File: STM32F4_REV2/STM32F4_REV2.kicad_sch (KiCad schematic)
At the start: 0 parts

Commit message: Uploading the PCB files
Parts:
- added C1, C2: 2u2, Package_QFP:LQFP-64_10x10mm_P0.5mm, symbol Device:C_Small
- added R1: 10k, Resistor_THT:R_Array_SIP4, symbol Device:R_Small
- added SW1: SW_SPDT, Button_Switch_SMD:SW_SPST_CK_KMS2xxGP, symbol Switch:SW_SPDT
- added U1: STM32F405RGT6, Package_QFP:LQFP-64_10x10mm_P0.5mm, symbol MCU_ST_STM32F4:STM32F405RGTx
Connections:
- new net: C2.1, U1.31 (VCAP_1)
- new net: R1.2, SW1.2 (B)
- new net: C1.1, U1.47 (VCAP_2)
- new net +3.3V: SW1.1 (A), U1.1 (VBAT), U1.19 (VDD), U1.32 (VDD), U1.48 (VDD), U1.64 (VDD)
- new net +3.3VA: U1.13 (VDDA)
- new net BOOT0: R1.1, U1.60 (BOOT0)
- new net GND: C1.2, C2.2, SW1.3 (C), U1.12 (VSSA), U1.18 (VSS), U1.63 (VSS)
- new net HSE_IN: U1.5 (PH0)
- new net HSE_OUT: U1.6 (PH1)
- new net NRST: U1.7 (NRST)
- new net SWDIO: U1.46 (PA13)
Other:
- company: (none) -> Quanttronix
- title: (none) -> STM32F4 Board

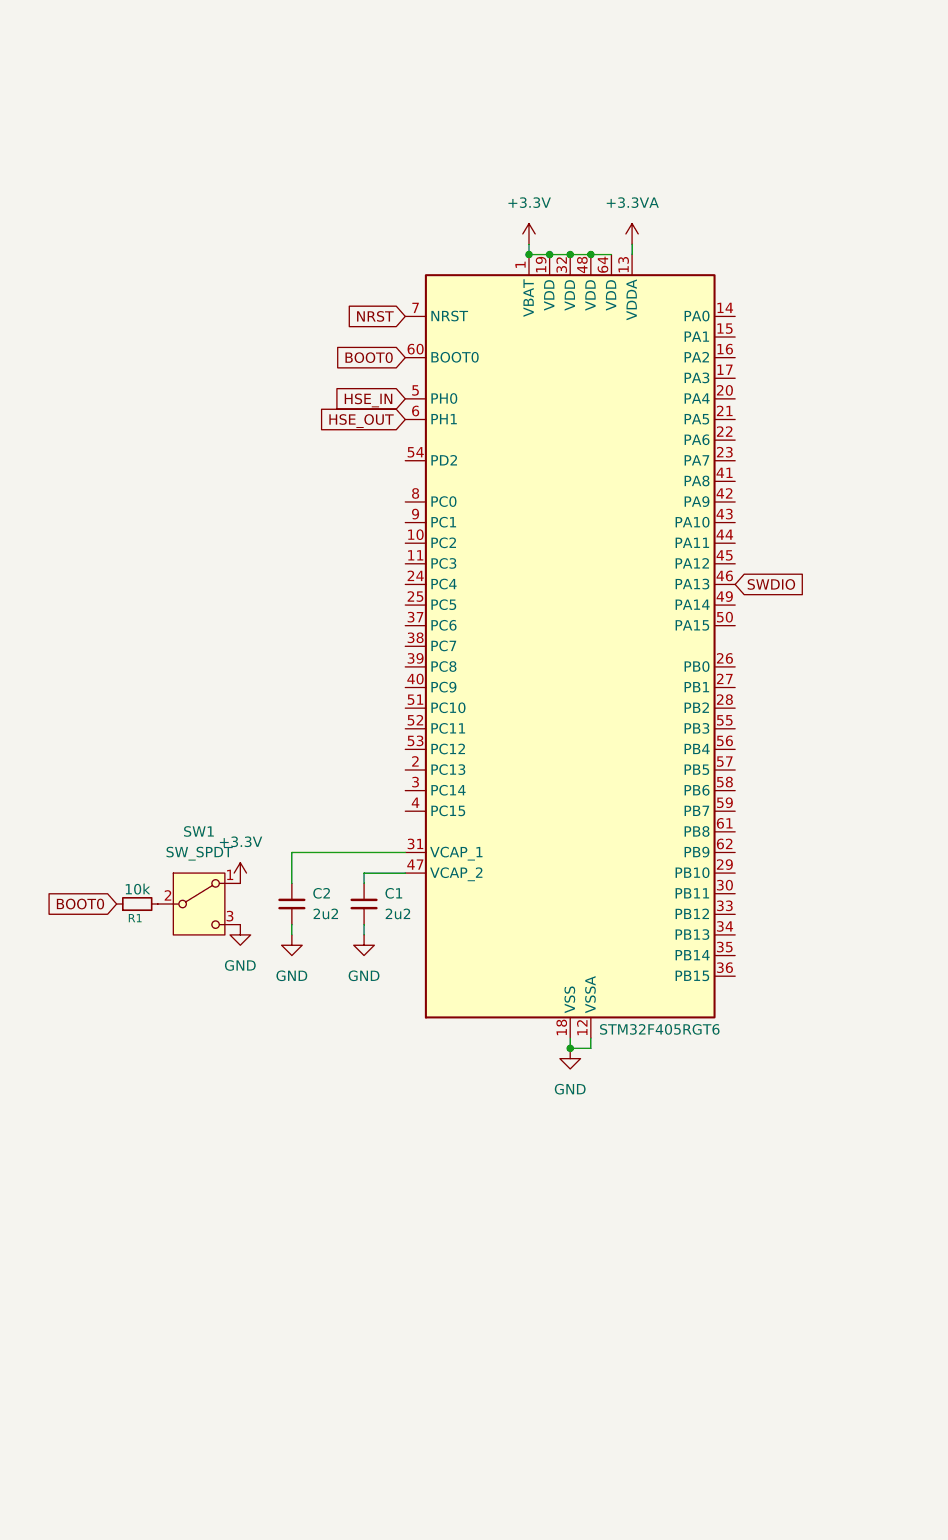
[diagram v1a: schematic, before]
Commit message: Updating the files
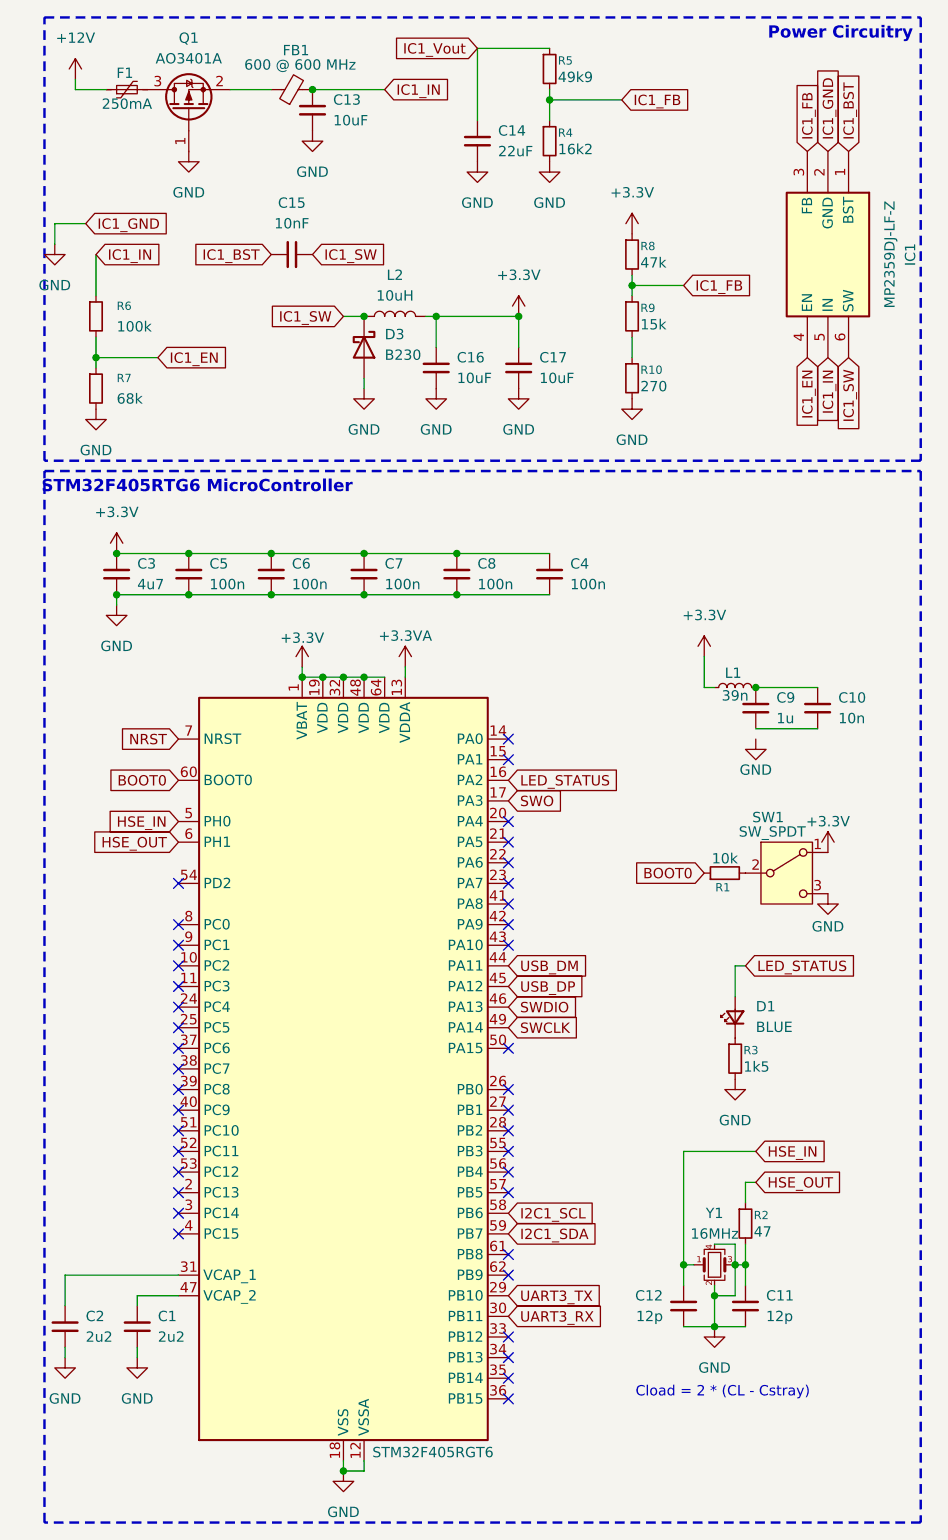
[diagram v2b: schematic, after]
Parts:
- added C10: 10n, symbol Device:C_Small
- added C11, C12: 12p, symbol Device:C_Small
- added C13, C16, C17: 10uF, symbol Device:C_Small
- added C14: 22uF, symbol Device:C_Small
- added C15: 10nF, symbol Device:C_Small
- added C3: 4u7, symbol Device:C_Small
- added C4, C5, C6, C7, C8: 100n, symbol Device:C_Small
- added C9: 1u, symbol Device:C_Small
- added D1: BLUE, symbol Device:LED_Small
- added D3: B230, Diode_SMD:D_SMB, symbol Diode:B230
- added F1: 250mA, symbol Device:Polyfuse_Small
- added FB1: 600 @ 600 MHz, Package_LCC:PLCC-84_29.3x29.3mm_P1.27mm, symbol Device:FerriteBead_Small
- added IC1: MP2359DJ-LF-Z, symbol SchmilliKiCADLibrary:MP2359DJ-LF-Z
- added L1: 39n, symbol Device:L_Small
- added L2: 10uH, Package_SON:WSON-8-1EP_6x5mm_P1.27mm_EP3.4x4mm, symbol Device:L
- added Q1: AO3401A, Package_TO_SOT_SMD:SOT-23, symbol Transistor_FET:AO3401A
- added R10: 270, symbol Device:R_Small
- added R2: 47, symbol Device:R_Small
- added R3: 1k5, symbol Device:R_Small
- added R4: 16k2, symbol Device:R_Small
- added R5: 49k9, symbol Device:R_Small
- added R6: 100k, symbol Device:R_Small
- added R7: 68k, symbol Device:R_Small
- added R8: 47k, symbol Device:R_Small
- added R9: 15k, symbol Device:R_Small
- added Y1: 16MHz, symbol Device:Crystal_GND24_Small
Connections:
- net +3.3V: now also C16.1, C17.1, C3.1, C4.1, C5.1, C6.1, C7.1, C8.1, L1.1, L2.2, R8.1
- net GND: now also C11.1, C11.2, C12.2, C13.2, C14.2, C16.2, C17.2, C3.2, C4.2, C5.2, C6.2, C7.2, C8.2, D3.2 (A), IC1.2 (GND), Q1.1 (G), R10.2, R2.2, R3.2, R4.2, R7.2, Y1.2 (G), Y1.3, Y1.4 (G)
- net HSE_IN: now also C12.1, Y1.1
- net HSE_OUT: now also R2.1
- net LED_STATUS: now reaches U1.16 (PA2)
- net LED_STATUS: now also D1.2 (A)
- net SWO: now reaches U1.17 (PA3)
- net UART3_TX: now reaches U1.29 (PB10)
- net UART3_RX: now reaches U1.30 (PB11)
- net USB_DM: now reaches U1.44 (PA11)
- net USB_DP: now reaches U1.45 (PA12)
- net SWCLK: now reaches U1.49 (PA14)
- net I2C1_SCL: now reaches U1.58 (PB6)
- net I2C1_SDA: now reaches U1.59 (PB7)
- new net: D1.1 (K), R3.1
- new net: C10.1, C9.1, L1.2
- new net: C10.2, C9.2
- new net: FB1.1, Q1.2 (S)
- new net: F1.2, Q1.3 (D)
- new net: R10.1, R9.2
- new net +12V: F1.1
- new net IC1_BST: C15.1, IC1.1 (BST)
- new net IC1_EN: IC1.4 (EN), R6.2, R7.1
- new net IC1_FB: IC1.3 (FB), R4.1, R5.2, R8.2, R9.1
- new net IC1_IN: C13.1, FB1.2, IC1.5 (IN), R6.1
- new net IC1_SW: C15.2, D3.1 (K), IC1.6 (SW), L2.1
- new net IC1_Vout: C14.1, R5.1
- no-connect marks 0 -> 39
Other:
- note added: "Cload = 2 * (CL - Cstray)"
- note added: "Power Circuitry"
- note added: "STM32F405RTG6 MicroController"
- moved on the sheet: C1, C2, R1, SW1

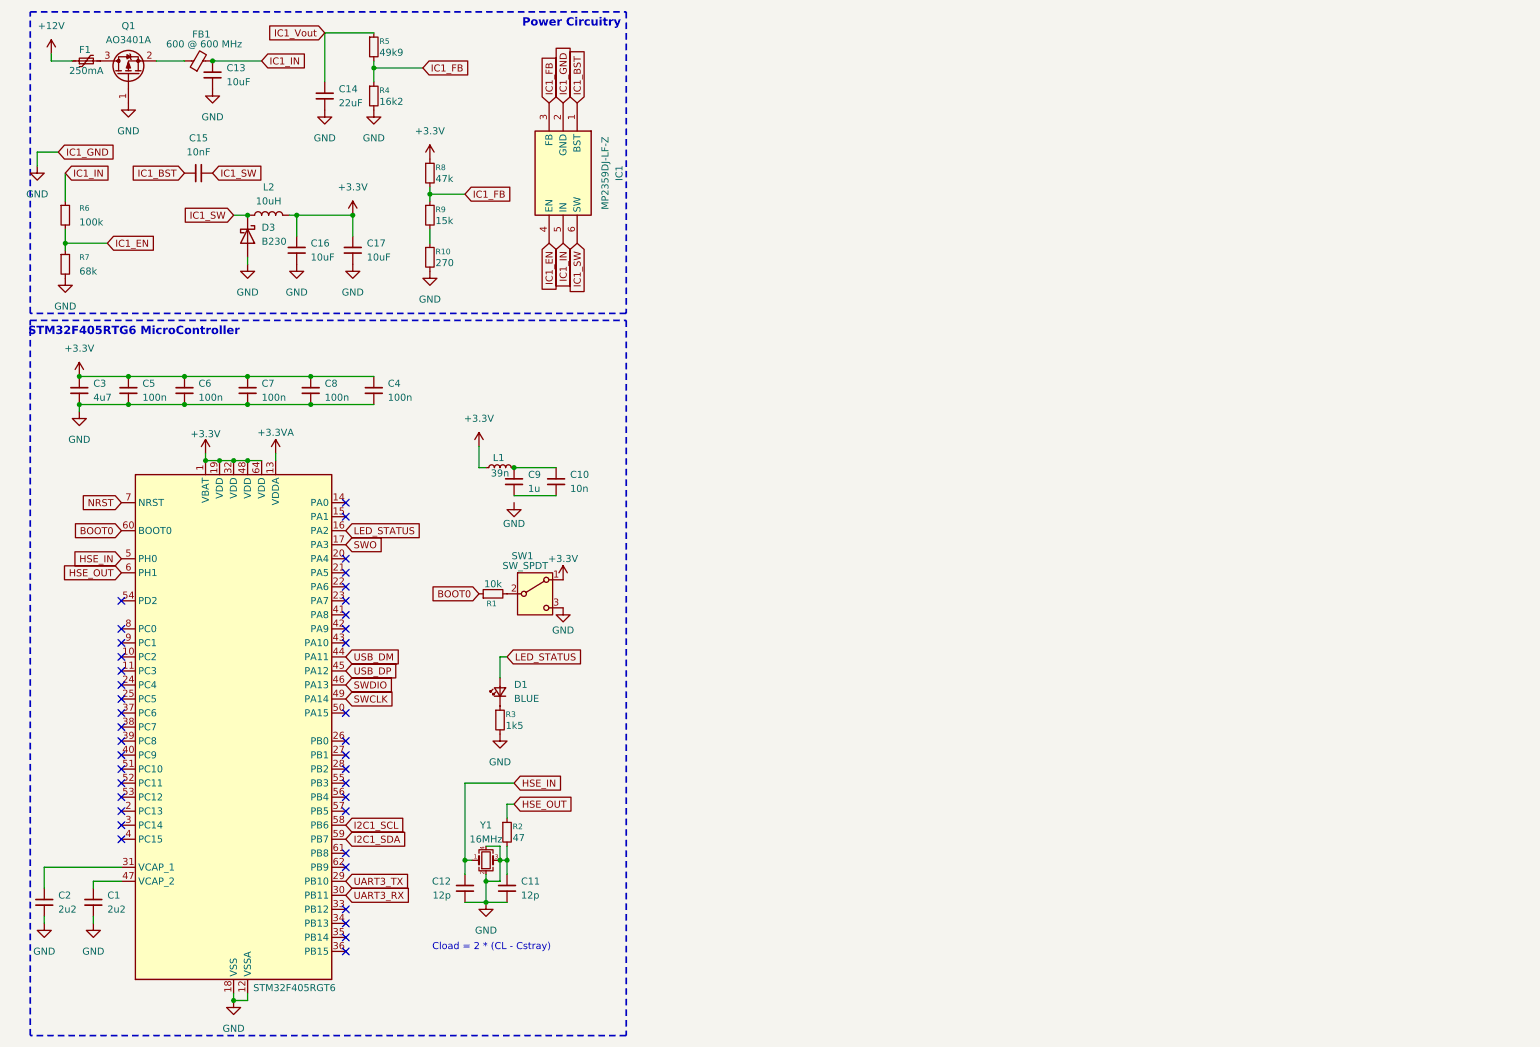
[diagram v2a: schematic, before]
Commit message: Uploading the PCB files
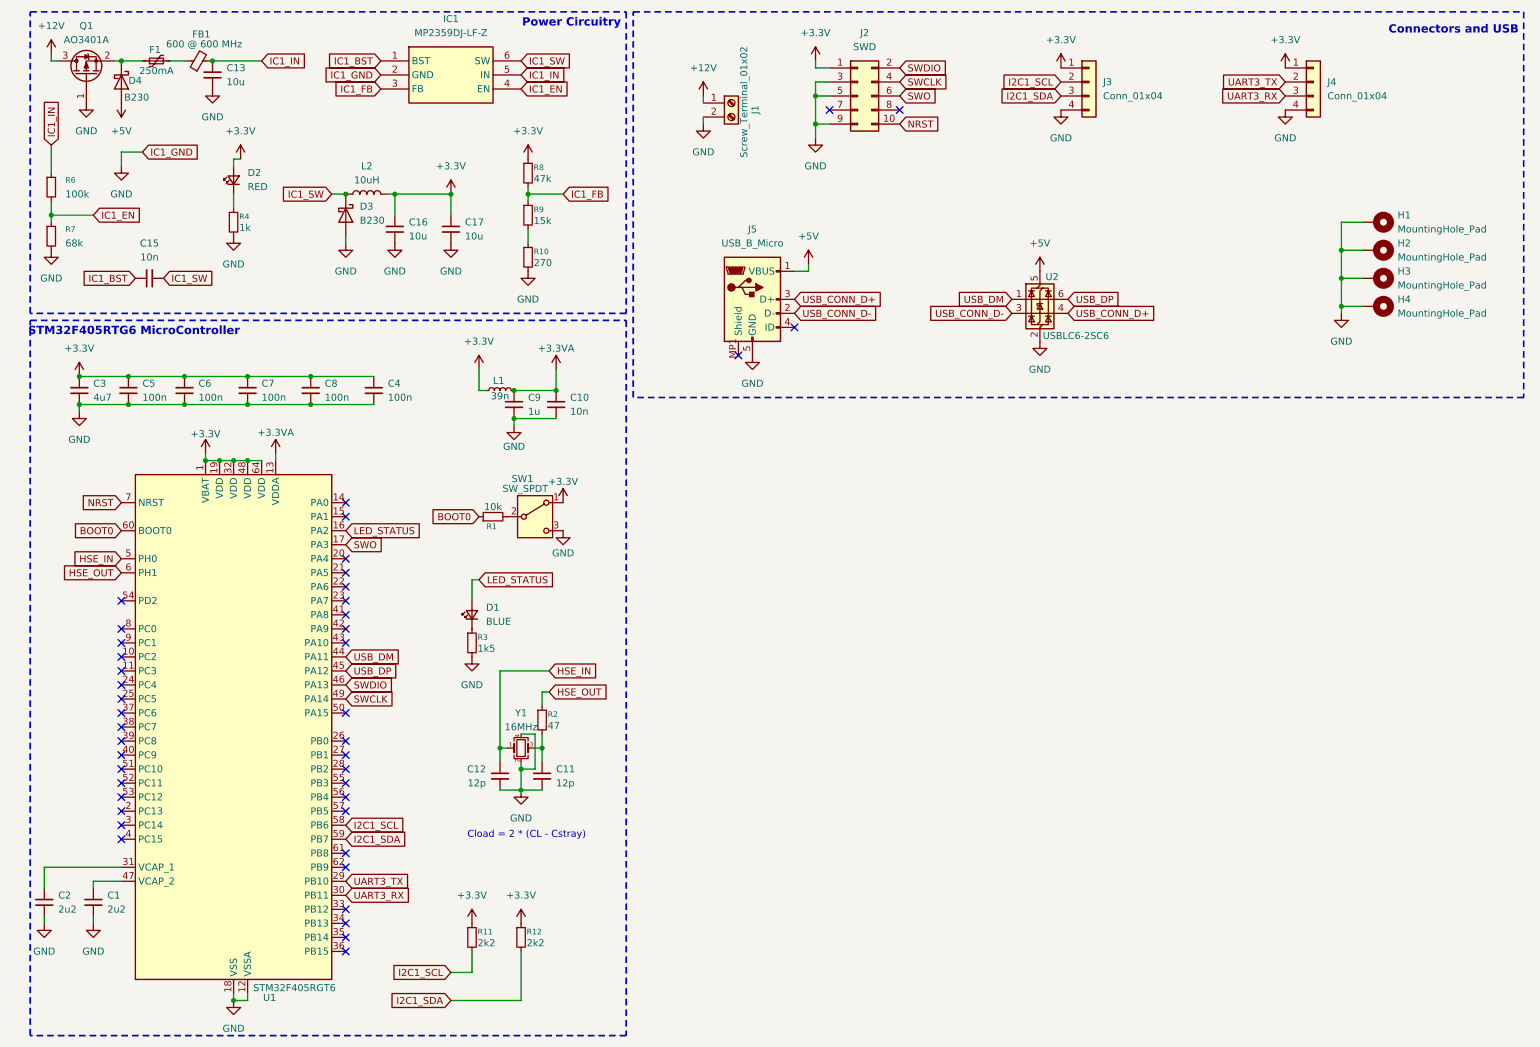
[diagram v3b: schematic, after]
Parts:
- removed C14: 22uF, symbol Device:C_Small
- removed IC1: MP2359DJ-LF-Z, symbol SchmilliKiCADLibrary:MP2359DJ-LF-Z
- removed R5: 49k9, symbol Device:R_Small
- added D2: RED, LED_SMD:LED_0603_1608Metric, symbol Device:LED_Small
- added D4: B230, Diode_SMD:D_SOD-123, symbol Diode:B230
- added H1, H2, H3, H4: MountingHole_Pad, MountingHole:MountingHole_4.3mm_M4_Pad_Via, symbol Mechanical:MountingHole_Pad
- added IC1: MP2359DJ-LF-Z, DownloadedLib:MP2359DJ-LF-Z, symbol DownloadedLib:MP2359DJ-LF-Z
- added J1: Screw_Terminal_01x02, TerminalBlock_Phoenix:TerminalBlock_Phoenix_PT-1,5-2-3.5-H_1x02_P3.50mm_Horizontal, symbol Connector:Screw_Terminal_01x02
- added J2: SWD, Connector_PinHeader_1.27mm:PinHeader_2x05_P1.27mm_Vertical_SMD, symbol Connector_Generic:Conn_02x05_Odd_Even
- added J3, J4: Conn_01x04, Connector_Molex:Molex_PicoBlade_53048-0410_1x04_P1.25mm_Horizontal, symbol Connector_Generic:Conn_01x04
- added J5: USB_B_Micro, DownloadedLib:101181930001LF, symbol Connector:USB_B_Micro
- added R11, R12: 2k2, Resistor_SMD:R_0402_1005Metric, symbol Device:R_Small
- added U2: USBLC6-2SC6, Package_TO_SOT_SMD:SOT-23-6, symbol Power_Protection:USBLC6-2SC6
- C1, C2: footprint Package_QFP:LQFP-64_10x10mm_P0.5mm -> Capacitor_SMD:C_0603_1608Metric
- C10, C11, C12, C4, C5, C6, C7, C8, C9: footprint (none) -> Capacitor_SMD:C_0402_1005Metric
- C13, C16, C17: value 10uF -> 10u; footprint (none) -> Capacitor_SMD:C_1206_3216Metric
- C15: value 10nF -> 10n; footprint (none) -> Capacitor_SMD:C_0603_1608Metric
- C3: footprint (none) -> Capacitor_SMD:C_0603_1608Metric
- D1: footprint (none) -> LED_SMD:LED_0603_1608Metric
- D3: footprint Diode_SMD:D_SMB -> Diode_SMD:D_SOD-123
- F1: footprint (none) -> Fuse:Fuse_1206_3216Metric
- FB1: footprint Package_LCC:PLCC-84_29.3x29.3mm_P1.27mm -> Capacitor_SMD:C_0805_2012Metric
- L1: footprint (none) -> Inductor_SMD:L_0402_1005Metric
- L2: footprint Package_SON:WSON-8-1EP_6x5mm_P1.27mm_EP3.4x4mm -> Inductor_SMD:L_Sunlord_MWSA0518S
- R1: footprint Resistor_THT:R_Array_SIP4 -> Resistor_SMD:R_0402_1005Metric
- R10, R3, R6, R7, R8, R9: footprint (none) -> Resistor_SMD:R_0603_1608Metric
- R2: footprint (none) -> Resistor_SMD:R_0402_1005Metric
- R4: value 16k2 -> 1k; footprint (none) -> Resistor_SMD:R_0603_1608Metric
- SW1: footprint Button_Switch_SMD:SW_SPST_CK_KMS2xxGP -> Button_Switch_SMD:SW_SPDT_PCM12
- Y1: footprint (none) -> Crystal:Crystal_SMD_3225-4Pin_3.2x2.5mm
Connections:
- net +12V: now also Q1.3 (D), J1.1 (Pin_1); no longer F1.1
- net +3.3V: now also D2.2 (A), J2.1 (Pin_1), J3.1 (Pin_1), J4.1 (Pin_1), R11.1, R12.1
- net +3.3VA: now also C10.1, C9.1, L1.2
- net GND: now also C10.2, C9.2, H1.1, H2.1, H3.1, H4.1, IC1.2 (GND), J1.2 (Pin_2), J2.3 (Pin_3), J2.5 (Pin_5), J2.9 (Pin_9), J3.4 (Pin_4), J4.4 (Pin_4), J5.5 (GND), U2.2 (GND); no longer C11.1, R2.2, Y1.3
- net I2C1_SCL: now also J3.2 (Pin_2), R11.2
- net I2C1_SDA: now also J3.3 (Pin_3), R12.2
- net IC1_BST: now also IC1.1 (BST)
- net IC1_EN: now also IC1.4 (EN)
- net IC1_FB: now also IC1.3 (FB); no longer R4.1
- net IC1_IN: now also IC1.5 (IN)
- net IC1_SW: now also IC1.6 (SW)
- net NRST: now also J2.10 (Pin_10)
- net SWCLK: now also J2.4 (Pin_4)
- net SWDIO: now also J2.2 (Pin_2)
- net SWO: now also J2.6 (Pin_6)
- net UART3_RX: now also J4.3 (Pin_3)
- net UART3_TX: now also J4.2 (Pin_2)
- net USB_DM: now also U2.1 (I/O1)
- net USB_DP: now also U2.6 (I/O1)
- net at Q1.2 (S): now also F1.1, D4.1 (K); no longer FB1.1
- net at F1.2: now also FB1.1; no longer Q1.3 (D)
- new net: C11.1, R2.2, Y1.3
- new net: D2.1 (K), R4.1
- new net +5V: D4.2 (A), J5.1 (VBUS), U2.5 (VBUS)
- new net USB_CONN_D+: J5.3 (D+), U2.4 (I/O2)
- new net USB_CONN_D-: J5.2 (D-), U2.3 (I/O2)
- no-connect marks 39 -> 43
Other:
- note added: "Connectors and USB"
- moved on the sheet: C10, C11, C12, C15, C16, C17, C9, D1, D3, F1, L1, L2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
